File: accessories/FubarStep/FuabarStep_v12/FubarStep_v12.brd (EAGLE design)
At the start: 115.3 x 54.6 mm, 82 parts, among them IC2 SN754410NE, IC3 SN754410NE, U1 FUBARINO_SD, U2 FUBARINO_MINI, U3 OKI-78SR-5/1.5-W36H-C, X1 DC21MMX

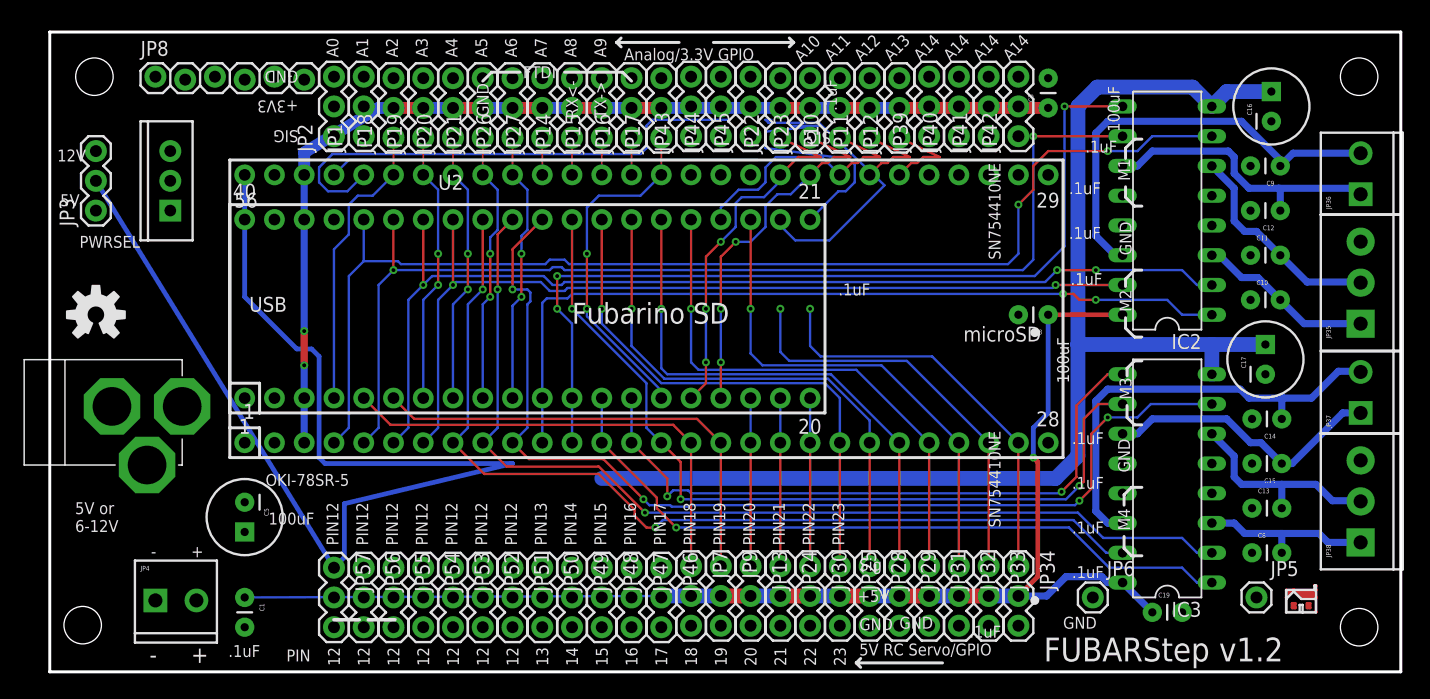
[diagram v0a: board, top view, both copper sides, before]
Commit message: New version of FubarStep - almost ready to go.
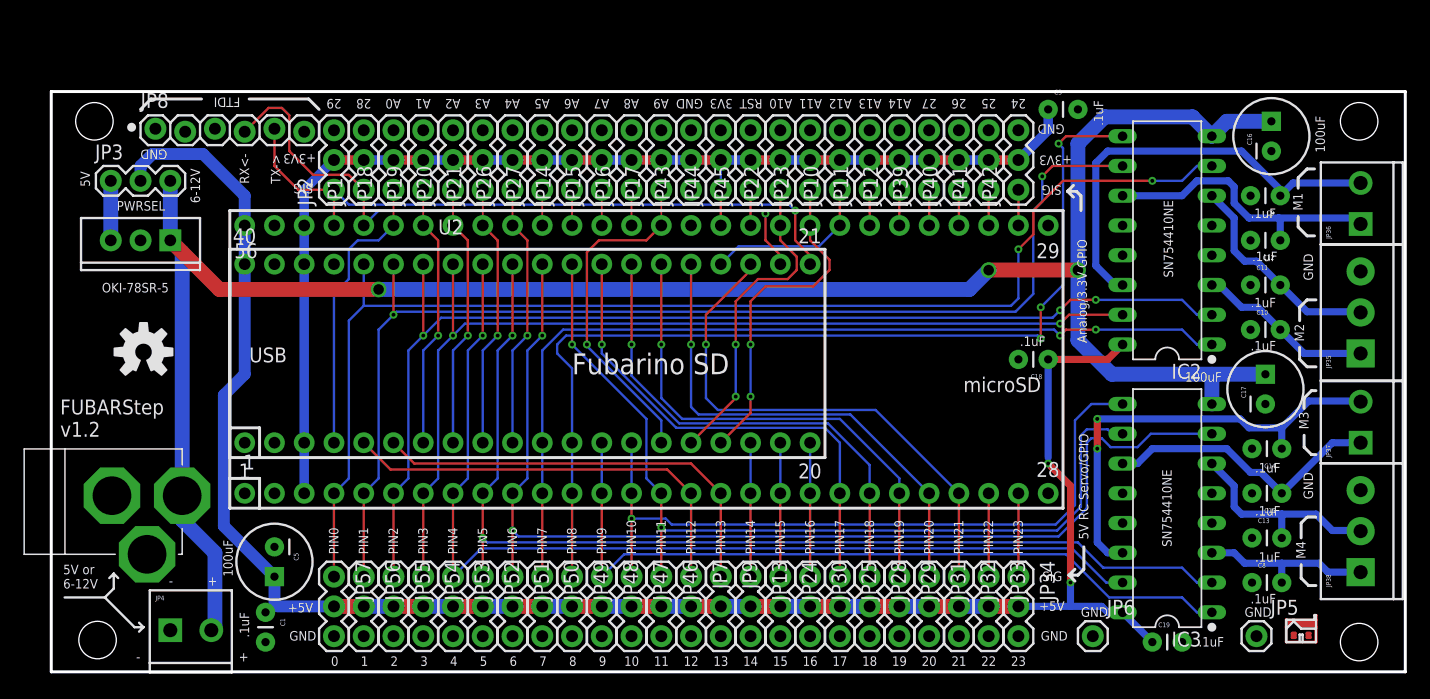
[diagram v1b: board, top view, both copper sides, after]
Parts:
- moved X1 7.62 mm to (4.83, 15.1)
- moved U3 5.68 mm to (7.62, 36.8), turned to 180 degrees
- moved LOGO1 5.16 mm to (7.87, 27.3)
- moved C5 4.58 mm to (19.1, 9.40)
- moved JP1 4.57 mm to (26.7, 41.1)
- moved JP2 4.57 mm to (24.1, 41.1)
- moved JP39 4.57 mm to (74.9, 41.1)
- moved JP40 4.57 mm to (77.5, 41.1)
- moved JP41 4.57 mm to (80.0, 41.1)
- moved JP42 4.57 mm to (82.5, 41.1)
- moved JP43 4.57 mm to (54.6, 41.1)
- moved JP44 4.57 mm to (57.1, 41.1)
- moved JP45 4.57 mm to (59.7, 41.1)
- moved JP10 4.45 mm to (67.3, 41.1)
- moved JP11 4.45 mm to (69.8, 41.1)
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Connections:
- removed net +3V3: U1.40
- new net PIN24: JP42.1, U1.30
- new net PIN25: JP41.1, U1.31
- new net PIN26: JP40.1, U1.32
- new net PIN27: JP39.1, U1.33
- net +5V: now also JP46.2, JP47.2, JP48.2, JP49.2, JP50.2, JP51.2, JP52.2, JP53.2, JP54.2, JP55.2, JP56.2, JP57.2
- net 3.3V: now also JP1.2, JP2.2, JP39.2, JP40.2, JP41.2, JP42.2, JP43.2, JP44.1, JP44.2, JP45.2, U1.40
- net GND: now also JP1.3, JP2.3, JP39.3, JP40.3, JP41.3, JP42.3, JP43.1, JP43.3, JP44.3, JP45.3, JP46.3, JP47.3, JP48.3, JP49.3, JP50.3, JP51.3, JP52.3, JP53.3, JP54.3, JP55.3, JP56.3, JP57.3
- net M1A1: now also JP55.1
- net M1A2: now also JP57.1
- net M1A3: now also JP56.1
- net M1A4: now also JP54.1
- net M1EN12: now also JP50.1
- net M1EN34: now also JP49.1
- net M2A1: now also JP52.1
- net M2A2: now also JP51.1
- net M2A3: now also JP46.1
- net M2A4: now also JP53.1
- net M2EN12: now also JP48.1
- net M2EN34: now also JP47.1
- net RESET: now also JP45.1
- net RX: now also JP1.1
- net TX: now also JP2.1
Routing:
- net VIN: track 108.2 -> 175.1 mm, vias 0 -> 3
- net +5V: track 214.7 -> 155.5 mm, vias 1 -> 2
- net PIN22: track 35.2 -> 7.11 mm, vias 1 -> 0
- net PIN23: track 34.9 -> 7.11 mm, vias 1 -> 0
- net RX: track 68.6 -> 58.5 mm, vias 0 -> 1
- net 3.3V: track 89.3 -> 98.9 mm, vias 2 -> 0
- net M1EN34: track 76.0 -> 85.3 mm
- net M1EN12: track 70.1 -> 78.1 mm
- net M1A1: track 89.1 -> 96.8 mm
- net M1A4: track 77.9 -> 85.6 mm
- net A12: track 22.2 -> 14.6 mm
- net M1A2: track 101.1 -> 108.7 mm
- net M1A3: track 93.5 -> 100.6 mm
- net M2EN34: track 56.6 -> 62.1 mm, vias 2 -> 1
- net M2A1: track 86.2 -> 91.5 mm
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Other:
- board size 115.3 x 54.6 mm -> 115.6 x 49.5 mm
- board text added: "0"
- board text added: "1"
- board text added: "10"
- board text added: "11"
- board text added: "2"
- board text added: "24"
- board text added: "25"
- board text added: "26"
- board text added: "27"
- board text added: "28"
- board text added: "29"
- board text added: "3"
- board text added: "3V3"
- board text added: "4"
- board text added: "5"
- board text added: "6"
- board text added: "6-12V"
- board text added: "7"
- board text added: "8"
- board text added: "9"
- board text added: "PIN0"
- board text added: "PIN1"
- board text added: "PIN10"
- board text added: "PIN11"
- board text added: "PIN2"
- board text added: "PIN3"
- board text added: "PIN4"
- board text added: "PIN5"
- board text added: "PIN6"
- board text added: "PIN7"
- board text added: "PIN8"
- board text added: "PIN9"
- board text added: "RST"
- board text removed: "12V"
- board text removed: "PIN"
- board text removed: "Sig"
